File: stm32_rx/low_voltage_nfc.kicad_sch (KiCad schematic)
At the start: 11 parts, among them U3 ST25R210-ANET, Y2 Crystal1

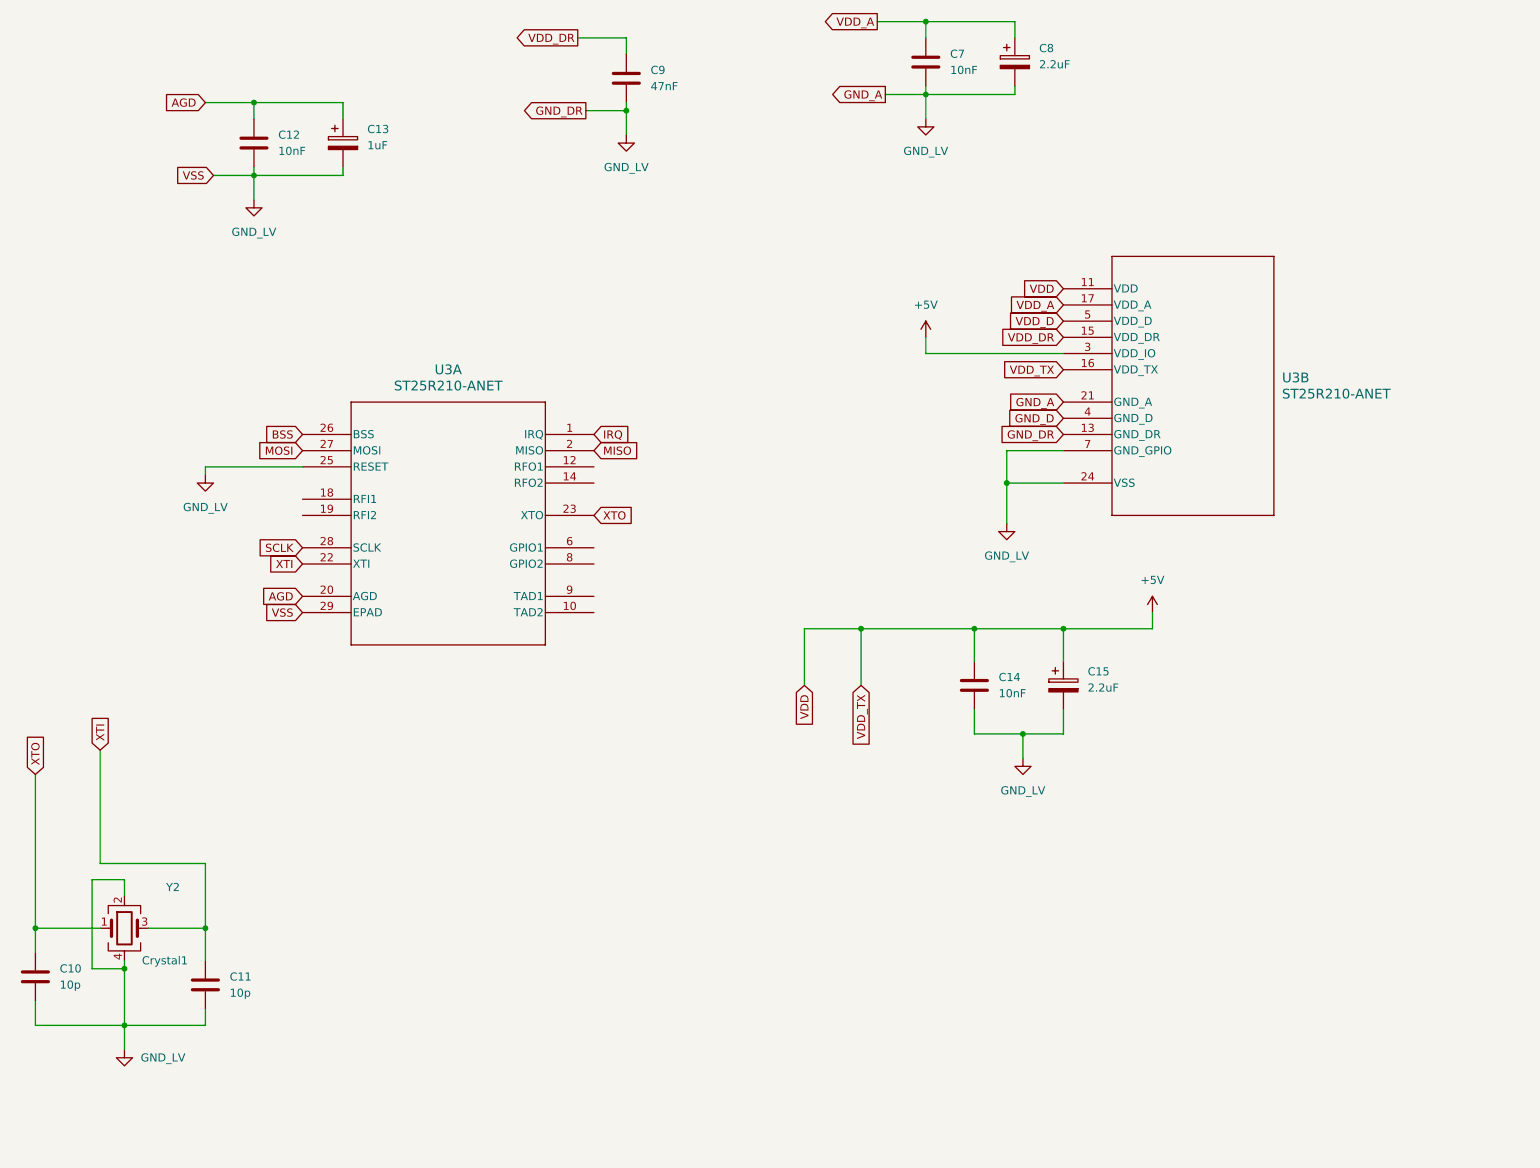
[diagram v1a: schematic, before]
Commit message: I can't find the right module
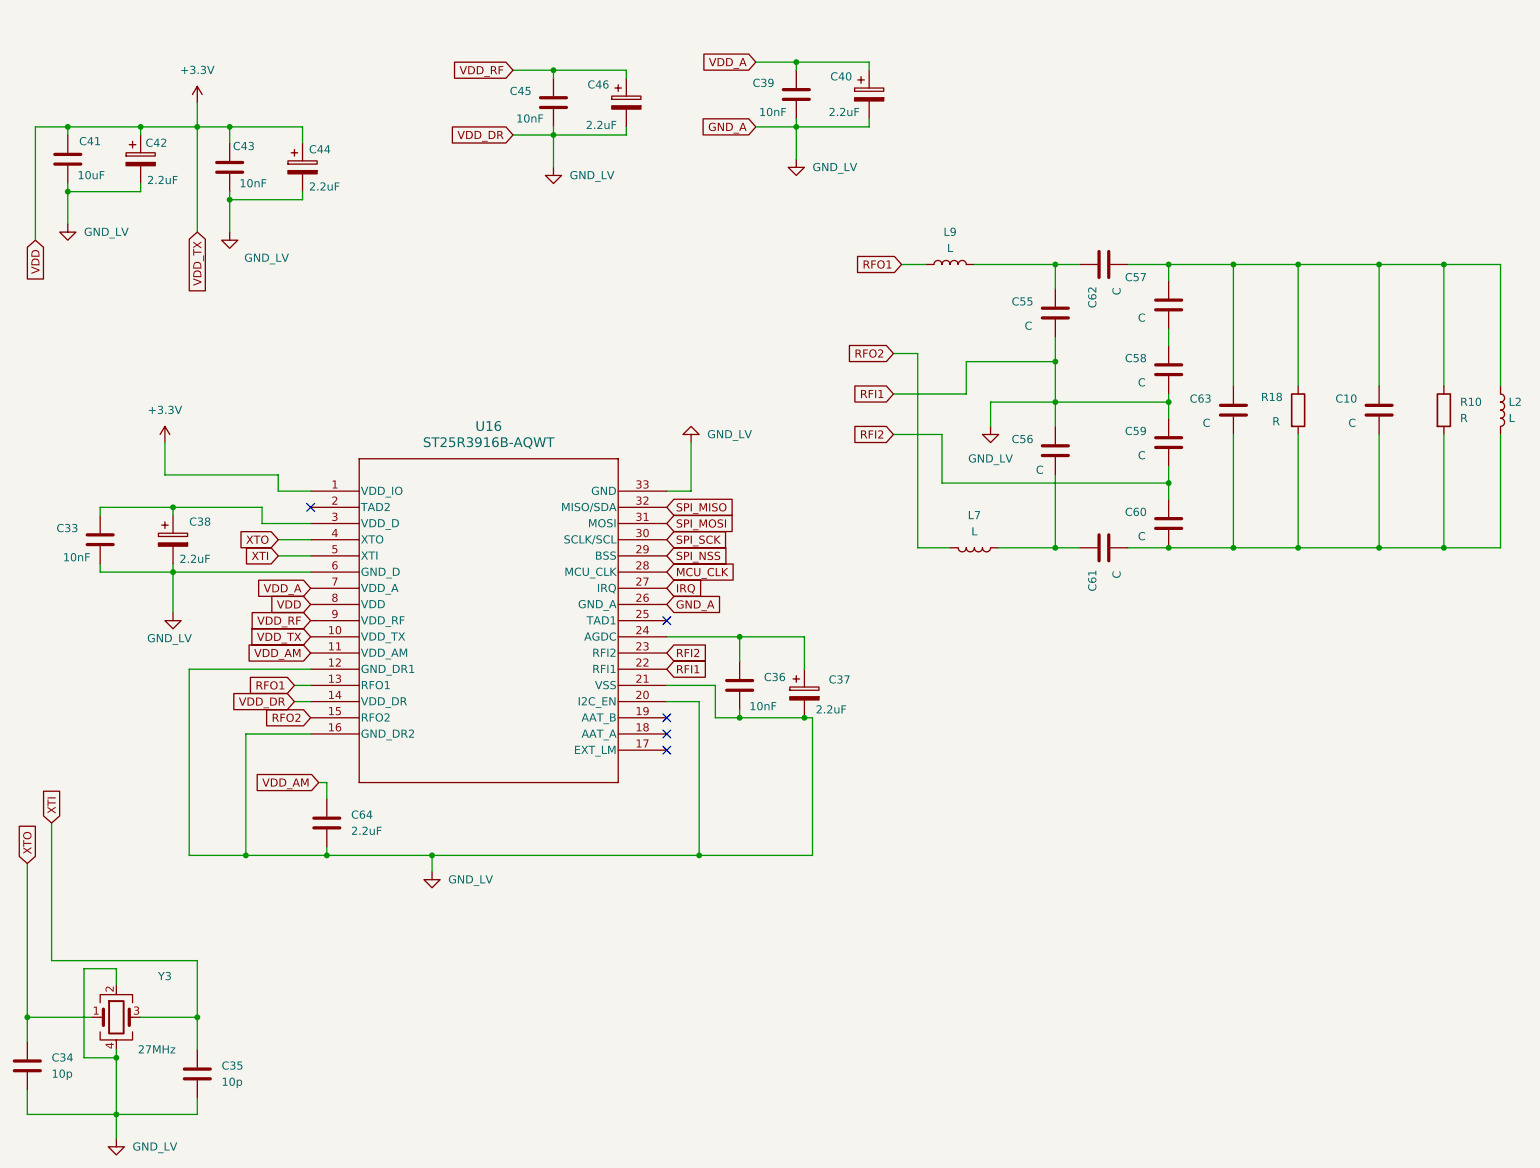
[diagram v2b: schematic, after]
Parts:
- removed C11: 10p, Capacitor_SMD:C_0402_1005Metric, symbol Device:C
- removed C12, C14, C7: 10nF, symbol Device:C
- removed C13: 1uF, symbol Device:C_Polarized
- removed C15, C8: 2.2uF, symbol Device:C_Polarized
- removed C9: 47nF, symbol Device:C
- removed U3: ST25R210-ANET, UFQFPN28_4X4_STM, symbol 2026-09-19_02-29-32:ST25R210-ANET
- removed Y2: Crystal1, Crystal:Crystal_SMD_3225-4Pin_3.2x2.5mm, symbol Device:Crystal_GND24
- added C33, C36, C39, C43, C45: 10nF, Capacitor_SMD:C_0402_1005Metric, symbol Device:C
- added C34, C35: 10p, Capacitor_SMD:C_0402_1005Metric, symbol Device:C
- added C37, C38, C40, C42, C44, C46: 2.2uF, Capacitor_SMD:C_0402_1005Metric, symbol Device:C_Polarized
- added C41: 10uF, Capacitor_SMD:C_0402_1005Metric, symbol Device:C
- added C55, C56, C57, C58, C59, C60, C61, C62, C63: C, symbol Device:C
- added C64: 2.2uF, Capacitor_SMD:C_0402_1005Metric, symbol Device:C
- added L2, L7, L9: L, symbol Device:L
- added R10, R18: R, symbol Device:R
- added U16: ST25R3916B-AQWT, WPT_TX:VFQFPN32_5X5_WETTABLE_STM, symbol 2026-09-17_02-59-22:ST25R3916B-AQWT
- added Y3: 27MHz, Crystal:Crystal_SMD_3225-4Pin_3.2x2.5mm, symbol Device:Crystal_GND24
- C10: value 10p -> C; footprint Capacitor_SMD:C_0402_1005Metric -> (none)
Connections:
- net GND_LV: now also C33.2, C34.2, C35.2, C36.2, C37.2, C38.2, C39.2, C40.2, C41.2, C42.2, C43.2, C44.2, C45.2, C46.2, C55.2, C56.1, C58.2, C59.1, C64.2, U16.12 (GND_DR1), U16.14 (VDD_DR), U16.16 (GND_DR2), U16.20 (I2C_EN), U16.21 (VSS), U16.22 (RFI1), U16.26 (GND_A), U16.33 (GND), U16.6 (GND_D), Y3.2, Y3.4; no longer C10.2
- net IRQ: now also U16.27 (IRQ)
- net VDD_A: now also C39.1, C40.1, U16.7 (VDD_A)
- net XTI: now also C35.1, U16.5 (XTI), Y3.3
- net XTO: now also C34.1, U16.4 (XTO), Y3.1; no longer C10.1
- new net: C57.2, C58.1
- new net: C10.1, C57.1, C62.2, C63.1, L2.1, R10.1, R18.1
- new net: C10.2, C60.2, C61.2, C63.2, L2.2, R10.2, R18.2
- new net: C36.1, C37.1, U16.24 (AGDC)
- new net: C33.1, C38.1, U16.3 (VDD_D)
- new net: C56.2, C61.1, L7.1
- new net: C55.1, C62.1, L9.2
- new net +3.3V: C41.1, C42.1, C43.1, C44.1, U16.1 (VDD_IO), U16.10 (VDD_TX), U16.8 (VDD)
- new net MCU_CLK: U16.28 (MCU_CLK)
- new net RFI2: C59.2, C60.1, U16.23 (RFI2)
- new net RFO1: L9.1, U16.13 (RFO1)
- new net RFO2: L7.2, U16.15 (RFO2)
- new net SPI_MISO: U16.32 (MISO/SDA)
- new net SPI_MOSI: U16.31 (MOSI)
- new net SPI_NSS: U16.29 (BSS)
- new net SPI_SCK: U16.30 (SCLK/SCL)
- new net VDD_AM: C64.1, U16.11 (VDD_AM)
- new net VDD_RF: C45.1, C46.1, U16.9 (VDD_RF)
- no-connect marks 0 -> 5
